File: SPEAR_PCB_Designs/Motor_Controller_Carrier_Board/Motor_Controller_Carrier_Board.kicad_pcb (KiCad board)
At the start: 2 copper layers, 104 x 47 mm, 17 parts, among them J1 Conn_01x02_Pin, J2 Conn_01x02_Pin, J3 Conn_01x02_Pin, J4 JST_S4B-XH-A-1, U1 AP63203WU

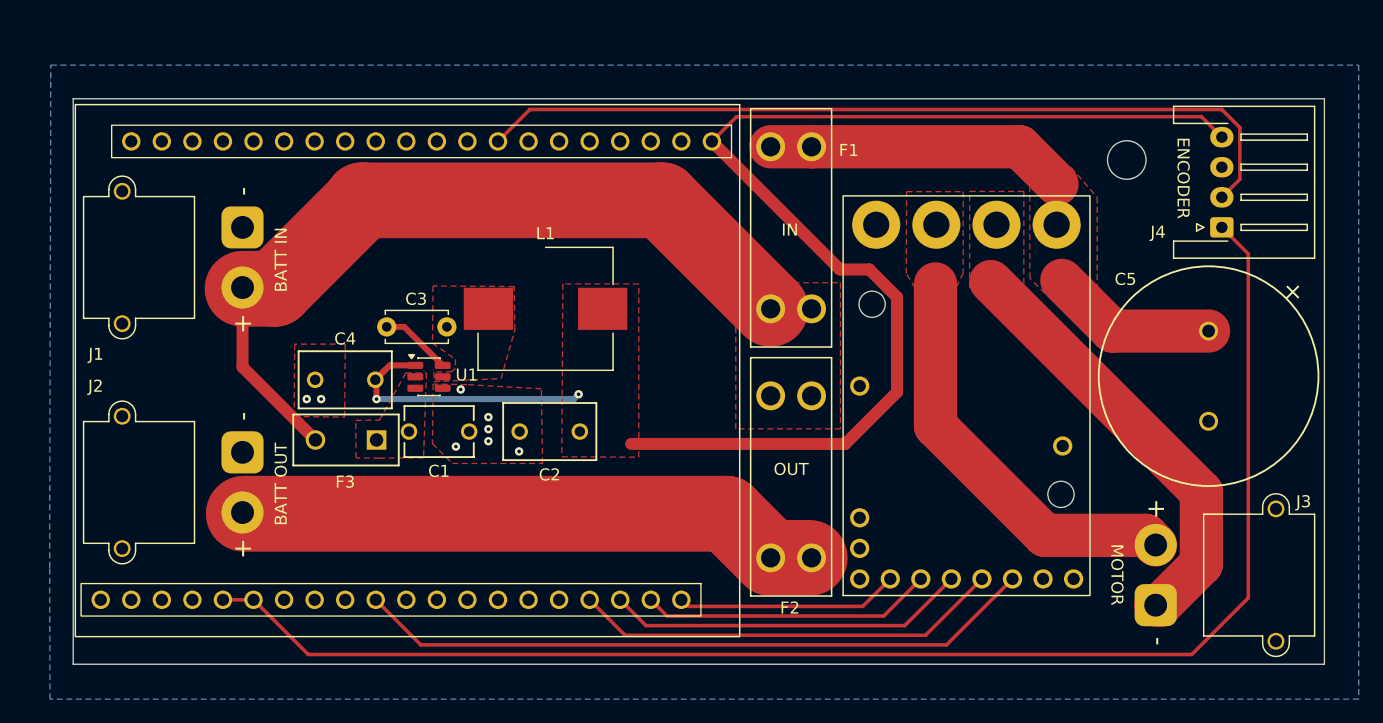
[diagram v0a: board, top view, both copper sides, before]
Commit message: Almost finished getting carrier board ready for fabrication
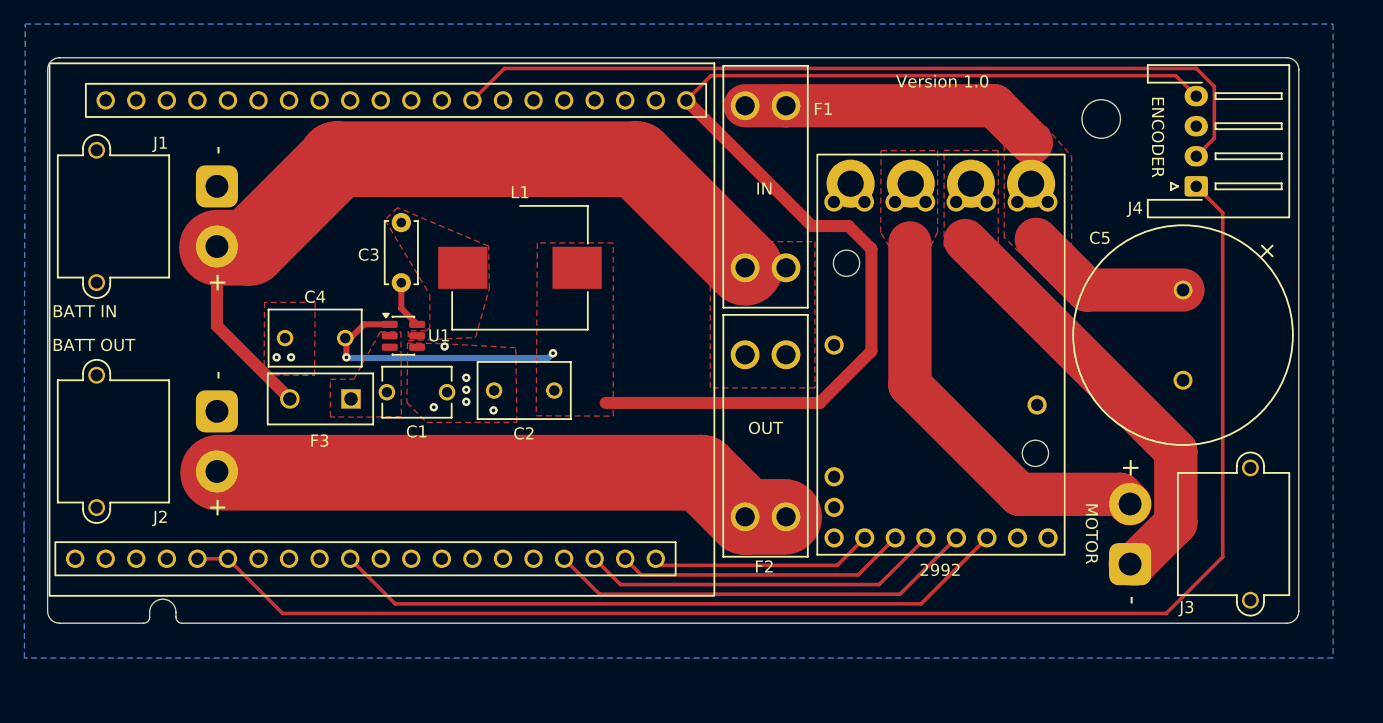
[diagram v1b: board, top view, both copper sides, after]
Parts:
- added G***: LOGO, SPEAR_Logos:spear_logo_10.0x10, B.Cu at (122.6, 80.3)
- C3: footprint Capacitor_THT:C_Disc_D5.0mm_W2.5mm_P5.00mm -> Motor_Controller_Carrier_Board:C_Disc_D5.0mm_W2.5mm_P5.00mm
- J1, J2, J3: footprint Connector_AMASS:AMASS_XT30PW-M_1x02_P2.50mm_Horizontal -> SPEAR_Connectors:AMASS_XT30PW-M_1x02_P2.50mm_Horizontal_1
- J4: footprint Connector_JST:JST_XH_S4B-XH-A-1_1x04_P2.50mm_Horizontal -> SPEAR_Connectors:JST_XH_S4B-XH-A-1_1x04_P2.50mm_Horizontal
- U1: footprint Package_TO_SOT_SMD:TSOT-23-6 -> Motor_Controller_Carrier_Board:TSOT-23-6
- moved C3 9.46 mm to (114.4, 82.7), turned to -90 degrees
- moved C4 4.28 mm to (109.7, 92.3)
- moved C5 4.02 mm to (179.4, 88.3)
- moved F1 4.02 mm to (144.7, 79.7)
- moved L1 4.02 mm to (124.3, 86.5)
- moved MDB1 4.02 mm to (149.1, 110.2)
- moved C2 4.02 mm to (127.1, 96.7)
- moved F2 4.02 mm to (144.7, 100.4)
- moved F3 4.02 mm to (110.2, 97.4)
- moved J1 4.02 mm to (99.1, 79.7)
- moved J2 4.02 mm to (99.1, 98.4)
- moved J3 4.02 mm to (175.0, 111.1)
- moved J4 4.02 mm to (180.5, 79.7)
- moved MCB1 4.02 mm to (140.3, 69.6)
- moved REF** 4.02 mm to (172.6, 74.1)
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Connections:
- MDB1 pad 12: Net-(J3-Pin_2) -> GND
- MDB1 pad 13: Net-(J3-Pin_1) -> GND
- MDB1 pad 14: /DRIVER_PWR -> GND
- MDB1 pad 16: GND -> Net-(J3-Pin_2)
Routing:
- net Net-(U1-BST): track 5.98 -> 4.00 mm
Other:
- outline, holes or cut-outs redrawn
- board text added: "2992"
- board text added: "Oliver Schneider Ronak Grover Henry Diep"
- board text added: "Version 1.0"
